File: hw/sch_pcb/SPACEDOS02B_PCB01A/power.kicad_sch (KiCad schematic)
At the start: 15 parts, among them J2 HEADER_2x01_PARALLEL, J3 HEADER_2x01_PARALLEL, U8 TPS613222ADBV

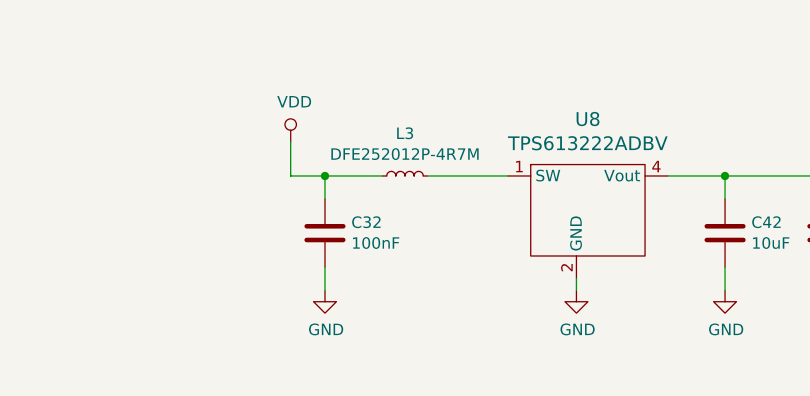
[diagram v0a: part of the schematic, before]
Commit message: Edit
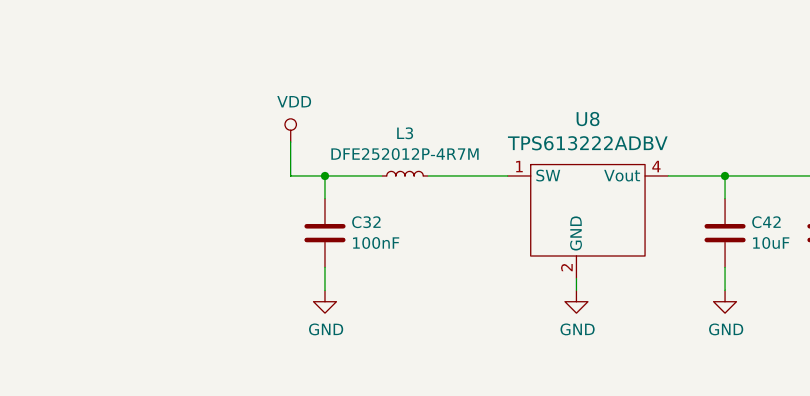
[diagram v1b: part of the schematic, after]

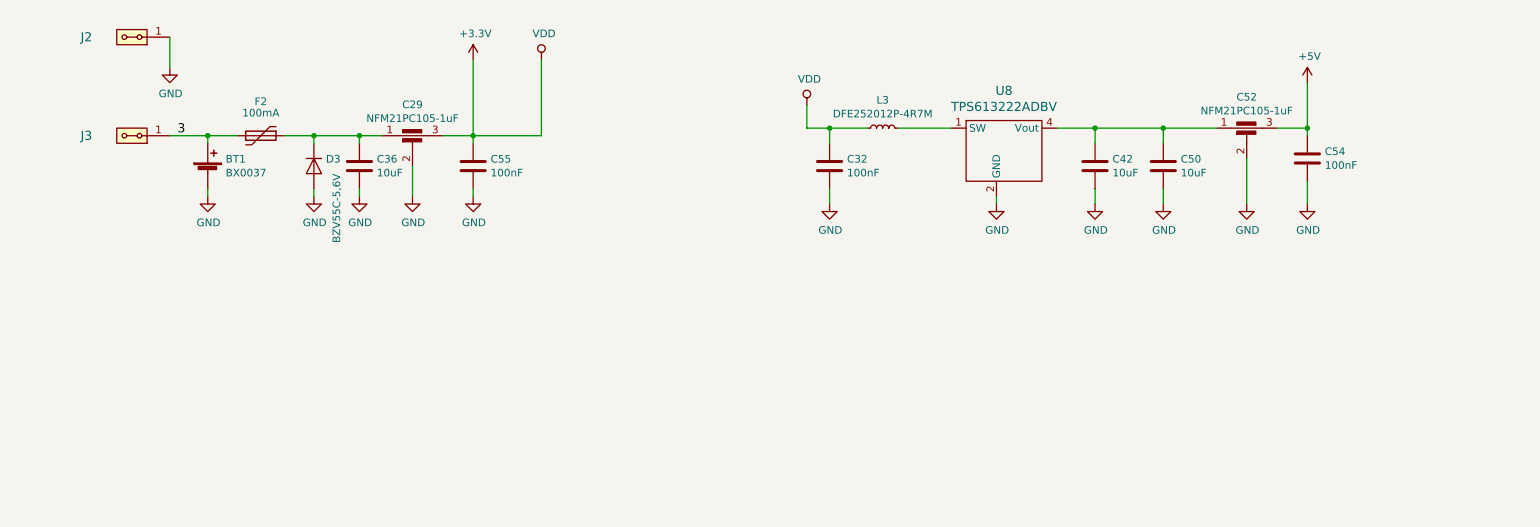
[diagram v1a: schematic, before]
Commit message: Edit schema
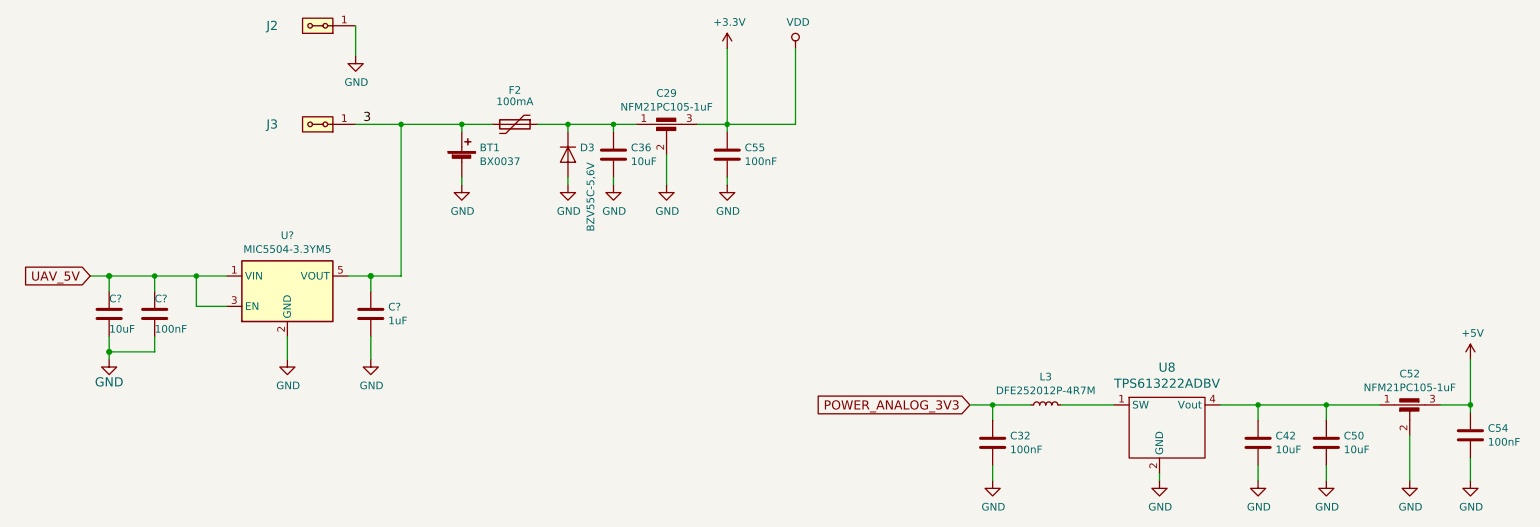
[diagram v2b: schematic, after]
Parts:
- added C?: 10uF, Mlab_R:SMD-0805, symbol Device:C
- added C?: 1uF, Mlab_R:SMD-0603, symbol Device:C
- added C?: 100nF, Mlab_R:SMD-0603, symbol Device:C
- added U?: MIC5504-3.3YM5, Package_TO_SOT_SMD:SOT-23-5, symbol Regulator_Linear:MIC5504-3.3YM5
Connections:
- net +3V3: no longer C32.1, L3.1
- net 3: now also C?.1, U?.5 (VOUT)
- net GND: now also C?.2, C?.2, C?.2, U?.2 (GND)
- new net POWER_ANALOG_3V3: C32.1, L3.1
- new net UAV_5V: C?.1, C?.1, U?.1 (VIN), U?.3 (EN)
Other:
- moved on the sheet: BT1, C29, C32, C36, C42, C50, C52, C54, C55, D3, F2, J2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
